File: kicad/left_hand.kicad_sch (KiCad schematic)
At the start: 31 parts, among them SW10 Gateron_ks_27, SW11 Gateron_ks_27, SW12 Gateron_ks_27, SW13 Gateron_ks_27, SW14 Gateron_ks_27, SW15 Gateron_ks_27, SW16 Gateron_ks_27, SW17 Gateron_ks_27, SW18 Gateron_ks_27, SW19 Gateron_ks_27, SW20 Gateron_ks_27, SW21 Gateron_ks_27, SW22 Gateron_ks_27, SW23 Gateron_ks_27, SW24 Gateron_ks_27, SW25 Gateron_ks_27, SW26 Gateron_ks_27, SW27 Gateron_ks_27, SW28 Gateron_ks_27, SW29 Gateron_ks_27, SW30 Gateron_ks_27, SW31 Gateron_ks_27, SW32 Gateron_ks_27, SW33 Gateron_ks_27, SW4 Gateron_ks_27, SW5 Gateron_ks_27, SW6 Gateron_ks_27, SW7 Gateron_ks_27, SW8 Gateron_ks_27, SW9 Gateron_ks_27, U2 74HC595

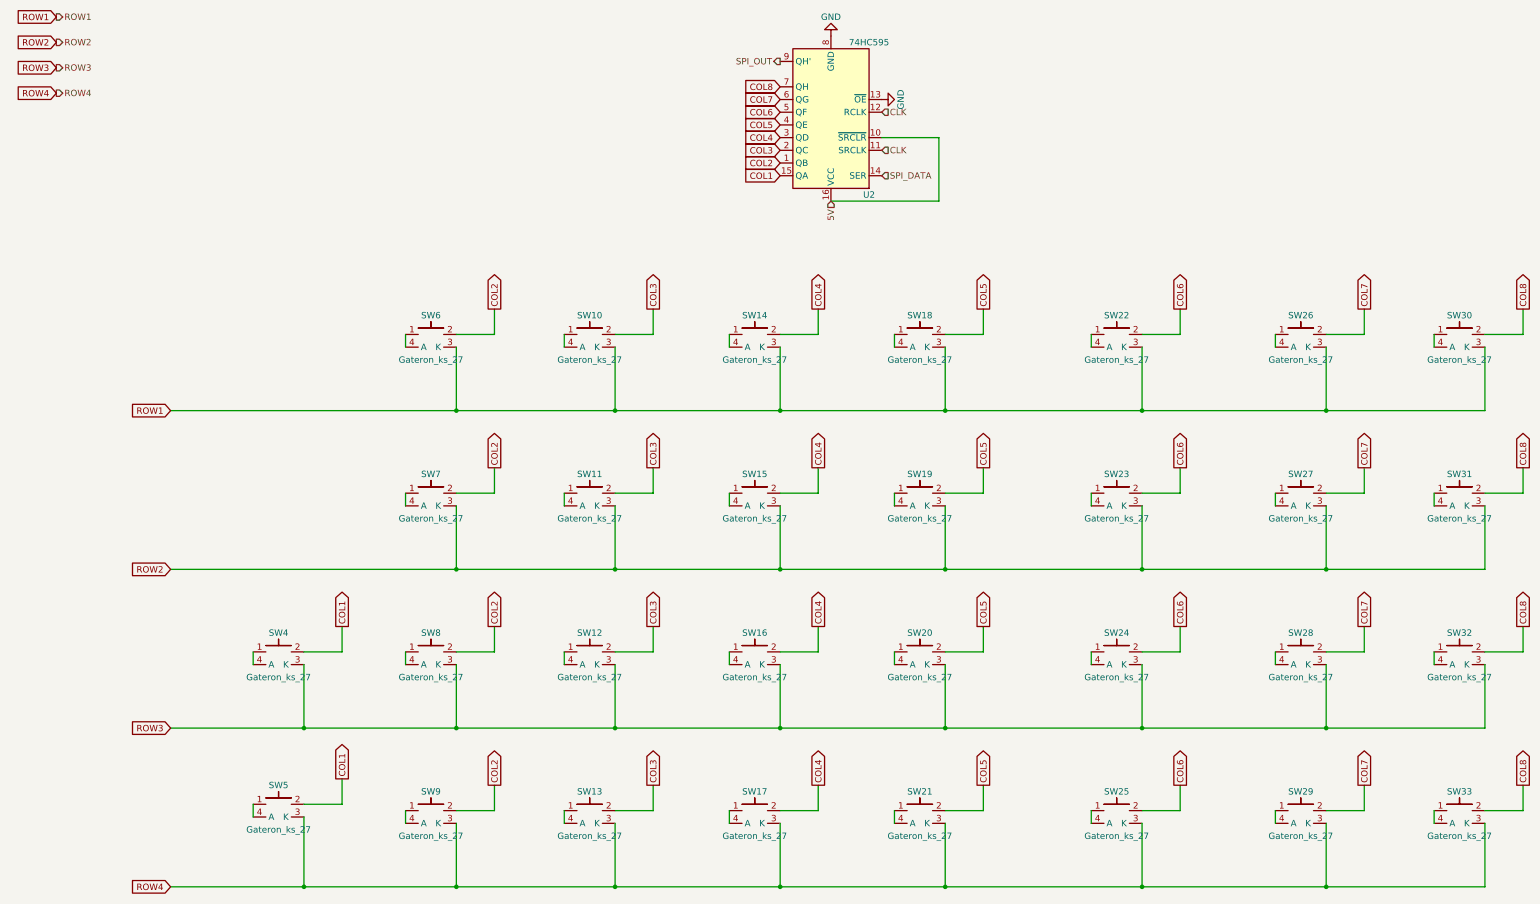
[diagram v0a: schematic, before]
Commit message: Update PCB
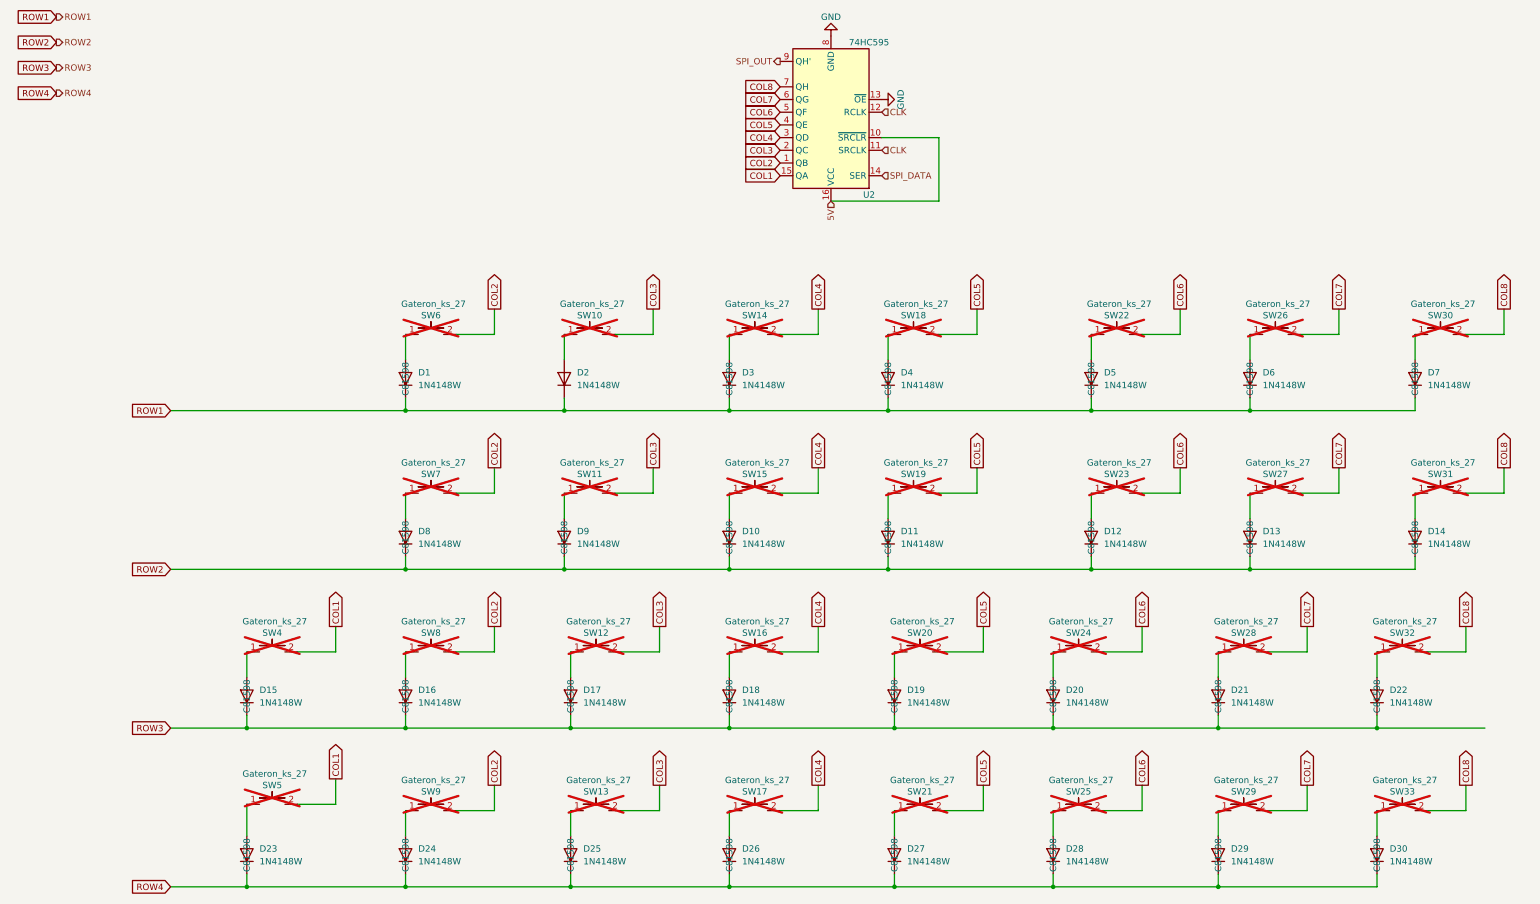
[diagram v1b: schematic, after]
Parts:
- added D1, D10, D11, D12, D13, D14, D15, D16, D17, D18, D19, D2, D20, D21, D22, D23, D24, D25, D26, D27, D28, D29, D3, D30, D4, D5, D6, D7, D8, D9: 1N4148W, Diode_SMD:D_SOD-123, symbol Diode:1N4148W-JLC
- SW10, SW11, SW12, SW13, SW14, SW15, SW16, SW17, SW18, SW19, SW20, SW21, SW22, SW23, SW24, SW25, SW26, SW27, SW28, SW29, SW30, SW31, SW32, SW33, SW4, SW5, SW6, SW7, SW8, SW9: now not fitted
- U2: LCSC (none) -> C72115
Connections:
- net ROW1: now also D1.1 (K), D2.1 (K), D3.1 (K), D4.1 (K), D5.1 (K), D6.1 (K), D7.1 (K); no longer SW10.3 (K), SW14.3 (K), SW18.3 (K), SW22.3 (K), SW26.3 (K), SW30.3 (K), SW6.3 (K)
- net ROW2: now also D10.1 (K), D11.1 (K), D12.1 (K), D13.1 (K), D14.1 (K), D8.1 (K), D9.1 (K); no longer SW11.3 (K), SW15.3 (K), SW19.3 (K), SW23.3 (K), SW27.3 (K), SW31.3 (K), SW7.3 (K)
- net ROW3: now also D15.1 (K), D16.1 (K), D17.1 (K), D18.1 (K), D19.1 (K), D20.1 (K), D21.1 (K), D22.1 (K); no longer SW12.3 (K), SW16.3 (K), SW20.3 (K), SW24.3 (K), SW28.3 (K), SW32.3 (K), SW4.3 (K), SW8.3 (K)
- net ROW4: now also D23.1 (K), D24.1 (K), D25.1 (K), D26.1 (K), D27.1 (K), D28.1 (K), D29.1 (K), D30.1 (K); no longer SW13.3 (K), SW17.3 (K), SW21.3 (K), SW25.3 (K), SW29.3 (K), SW33.3 (K), SW5.3 (K), SW9.3 (K)
- net at SW27.1: now also D13.2 (A); no longer SW27.4 (A)
- net at SW15.1: now also D10.2 (A); no longer SW15.4 (A)
- net at SW19.1: now also D11.2 (A); no longer SW19.4 (A)
- net at SW13.1: now also D25.2 (A); no longer SW13.4 (A)
- net at SW22.1: now also D5.2 (A); no longer SW22.4 (A)
- net at SW5.1: now also D23.2 (A); no longer SW5.4 (A)
- net at SW30.1: now also D7.2 (A); no longer SW30.4 (A)
- net at SW24.1: now also D20.2 (A); no longer SW24.4 (A)
- net at SW33.1: now also D30.2 (A); no longer SW33.4 (A)
- net at SW28.1: now also D21.2 (A); no longer SW28.4 (A)
- net at SW4.1: now also D15.2 (A); no longer SW4.4 (A)
- net at SW23.1: now also D12.2 (A); no longer SW23.4 (A)
- net at SW26.1: now also D6.2 (A); no longer SW26.4 (A)
- net at SW17.1: now also D26.2 (A); no longer SW17.4 (A)
- net at SW18.1: now also D4.2 (A); no longer SW18.4 (A)
- net at SW7.1: now also D8.2 (A); no longer SW7.4 (A)
- net at SW11.1: now also D9.2 (A); no longer SW11.4 (A)
- net at SW29.1: now also D29.2 (A); no longer SW29.4 (A)
- net at SW31.1: now also D14.2 (A); no longer SW31.4 (A)
- net at SW6.1: now also D1.2 (A); no longer SW6.4 (A)
- net at SW25.1: now also D28.2 (A); no longer SW25.4 (A)
- net at SW20.1: now also D19.2 (A); no longer SW20.4 (A)
- net at SW9.1: now also D24.2 (A); no longer SW9.4 (A)
- net at SW16.1: now also D18.2 (A); no longer SW16.4 (A)
- net at SW8.1: now also D16.2 (A); no longer SW8.4 (A)
- net at SW10.1: now also D2.2 (A); no longer SW10.4 (A)
- net at SW21.1: now also D27.2 (A); no longer SW21.4 (A)
- net at SW12.1: now also D17.2 (A); no longer SW12.4 (A)
- net at SW14.1: now also D3.2 (A); no longer SW14.4 (A)
- net at SW32.1: now also D22.2 (A); no longer SW32.4 (A)
